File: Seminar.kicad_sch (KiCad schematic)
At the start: 17 parts, among them SW1 SW_Push, SW2 SW_Push, U1 NUCLEO64-F446RE, U2 PCF8574AP

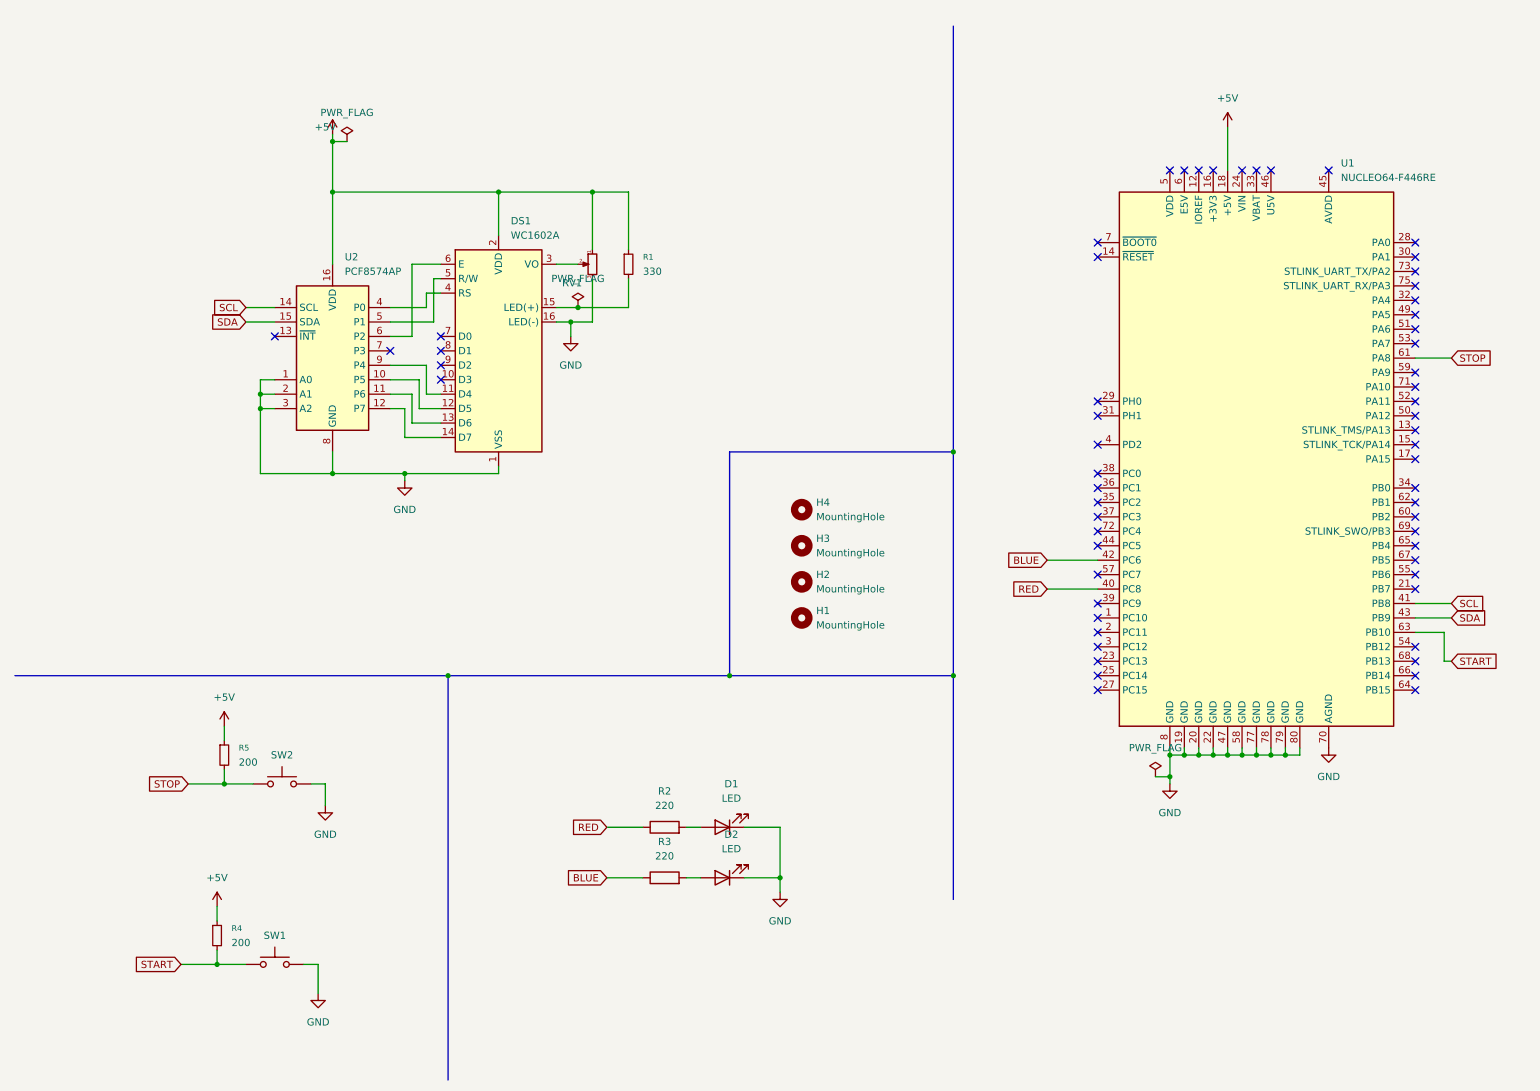
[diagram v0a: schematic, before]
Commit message: Update Seminar 7.12.
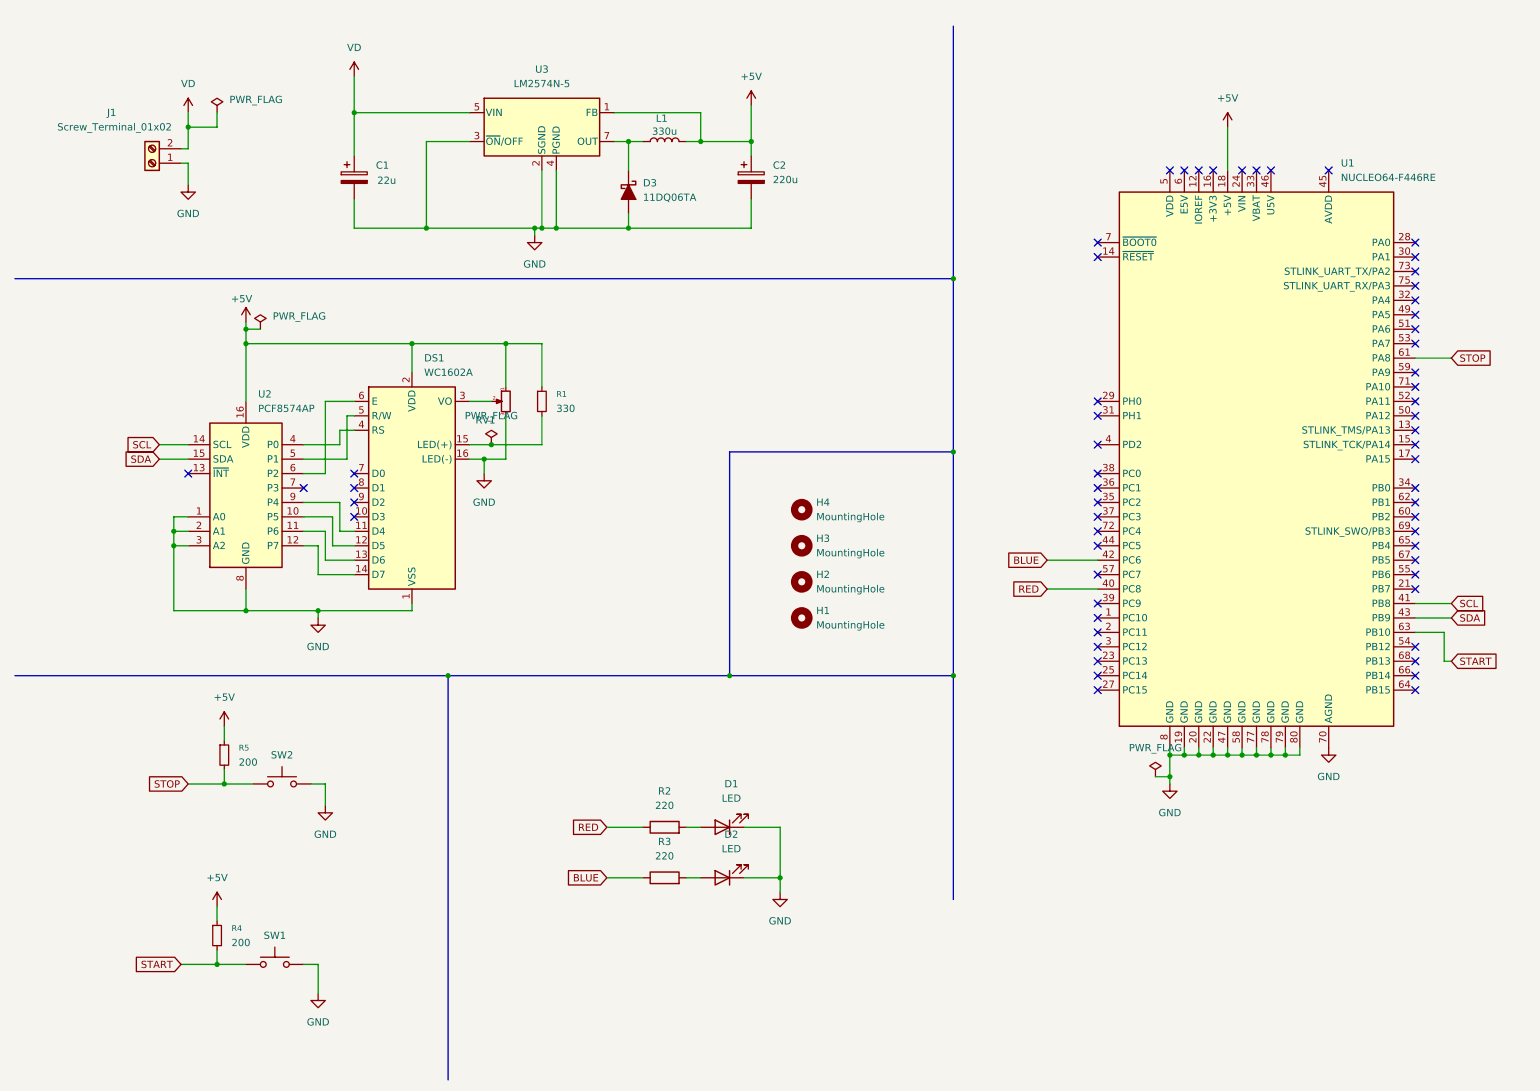
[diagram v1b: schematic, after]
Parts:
- added C1: 22u, Capacitor_THT:CP_Radial_D5.0mm_P2.00mm, symbol Device:C_Polarized
- added C2: 220u, Capacitor_THT:CP_Radial_D5.0mm_P2.00mm, symbol Device:C_Polarized
- added D3: 11DQ06TA, Diode_THT:D_DO-41_SOD81_P12.70mm_Horizontal, symbol Device:D_Schottky_Filled
- added J1: Screw_Terminal_01x02, TerminalBlock_MetzConnect:TerminalBlock_MetzConnect_Type011_RT05502HBLC_1x02_P5.00mm_Horizontal, symbol Connector:Screw_Terminal_01x02
- added L1: 330u, Inductor_THT:L_Radial_D7.2mm_P3.00mm_Murata_1700, symbol Device:L
- added U3: LM2574N-5, Package_DIP:DIP-8_W7.62mm, symbol Regulator_Switching:LM2574N-5
- DS1: Manufacturer (none) -> Wandisplay; Manufacturer part number (none) -> WC1602B0SGW6B-A1
- U1: Manufacturer (none) -> STMicroelectronics; Manufacturer part number (none) -> STM32F446RET6
- U2: Manufacturer (none) -> NXP; Manufacturer part number (none) -> PCF8574AP,112
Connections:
- net +5V: now also C2.1, L1.2, U3.1 (FB)
- net GND: now also C1.2, C2.2, D3.2 (A), J1.1 (Pin_1), U3.2 (SGND), U3.3 (~{ON}/OFF), U3.4 (PGND)
- new net: D3.1 (K), L1.1, U3.7 (OUT)
- new net VD: C1.1, J1.2 (Pin_2), U3.5 (VIN)
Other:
- moved on the sheet: DS1, R1, RV1, U2

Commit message: Update Seminar 7.12. dva
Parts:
- RV1: footprint Potentiometer_SMD:Potentiometer_ACP_CA6-VSMD_Vertical -> Potentiometer_THT:Potentiometer_Bourns_3299Y_Vertical
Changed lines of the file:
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@@
 			)
 		)
-		(property "Footprint" "Potentiometer_SMD:Potentiometer_ACP_CA6-VSMD_Vertical"
+		(property "Footprint" "Potentiometer_THT:Potentiometer_Bourns_3299Y_Vertical"
 			(at 99.06 78.74 0)
 			(effects

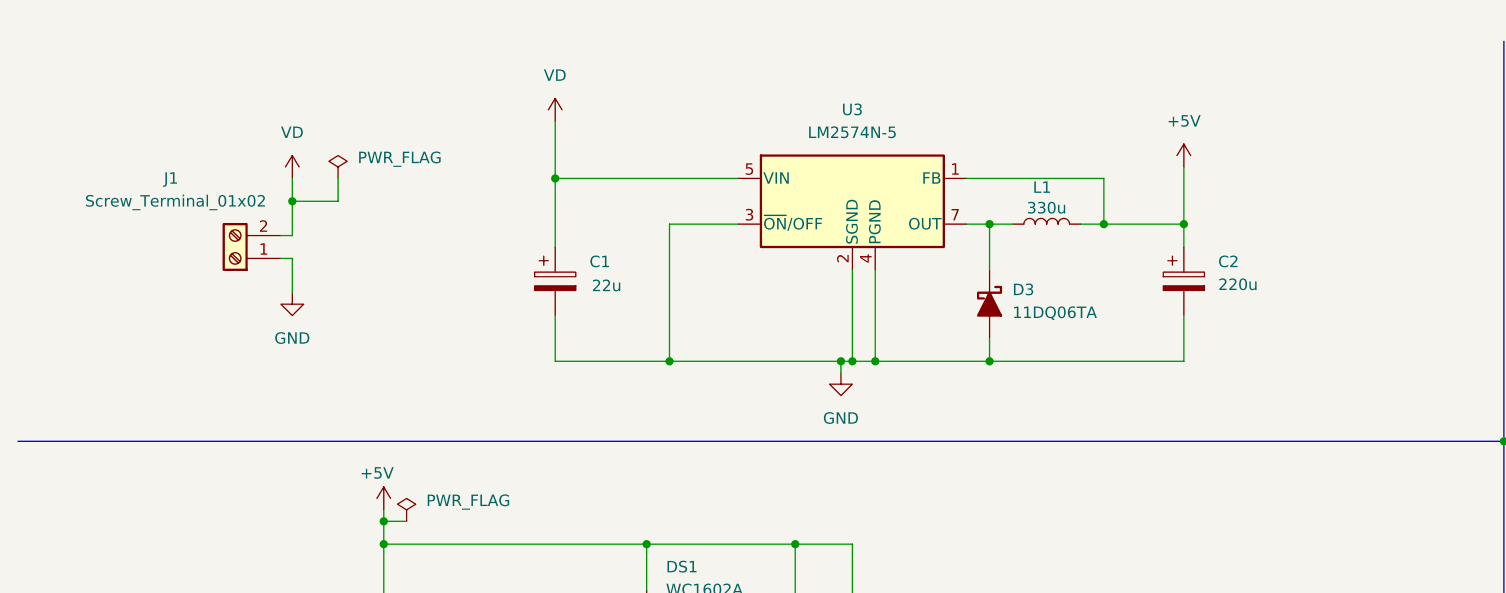
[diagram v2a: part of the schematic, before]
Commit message: Baterija i Step up
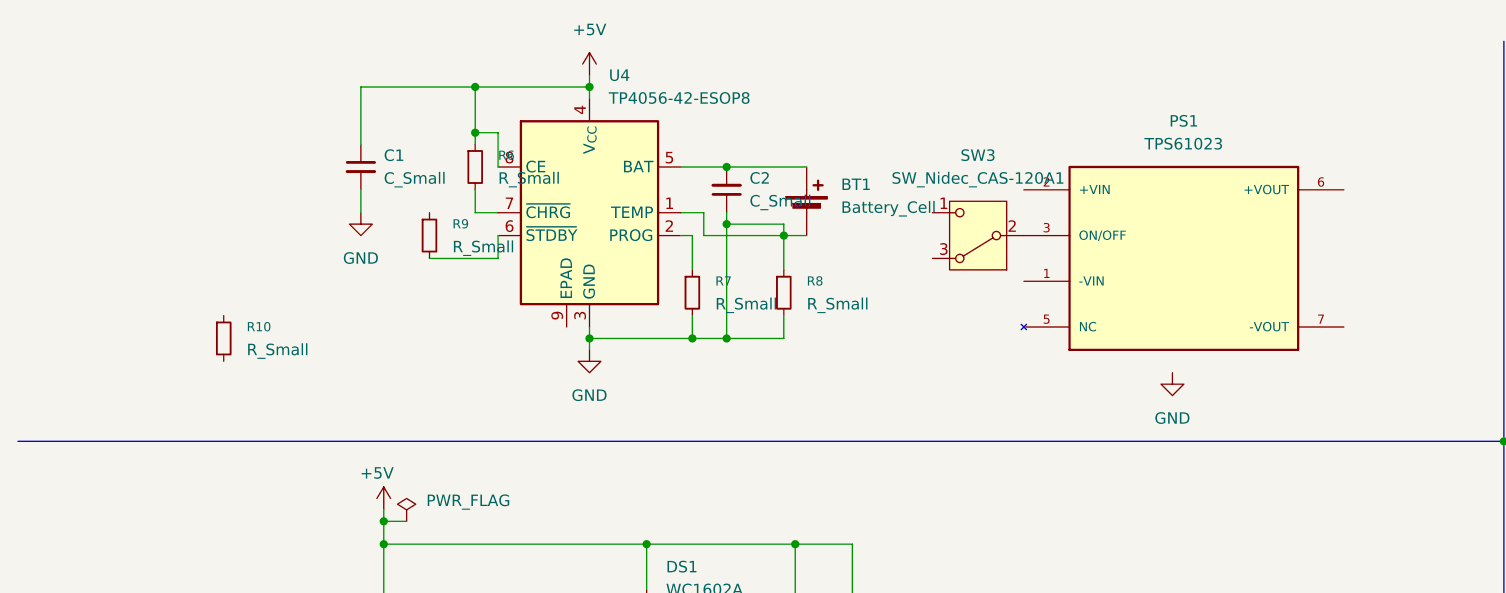
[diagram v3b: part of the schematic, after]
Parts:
- removed C1: 22u, Capacitor_THT:CP_Radial_D5.0mm_P2.00mm, symbol Device:C_Polarized
- removed C2: 220u, Capacitor_THT:CP_Radial_D5.0mm_P2.00mm, symbol Device:C_Polarized
- removed D3: 11DQ06TA, Diode_THT:D_DO-41_SOD81_P12.70mm_Horizontal, symbol Device:D_Schottky_Filled
- removed J1: Screw_Terminal_01x02, TerminalBlock_MetzConnect:TerminalBlock_MetzConnect_Type011_RT05502HBLC_1x02_P5.00mm_Horizontal, symbol Connector:Screw_Terminal_01x02
- removed L1: 330u, Inductor_THT:L_Radial_D7.2mm_P3.00mm_Murata_1700, symbol Device:L
- removed U3: LM2574N-5, Package_DIP:DIP-8_W7.62mm, symbol Regulator_Switching:LM2574N-5
- added BT1: Battery_Cell, symbol Device:Battery_Cell
- added C1, C2: C_Small, symbol Device:C_Small
- added PS1: TPS61023, CONV_PDQ2-D5-S3-S:CONV_PDQ2-D5-S3-S, symbol PDQ2-D5-S3-S:PDQ2-D5-S3-S
- added R10, R6, R7, R8, R9: R_Small, symbol Device:R_Small
- added SW3: SW_Nidec_CAS-120A1, Button_Switch_SMD:Nidec_Copal_CAS-120A, symbol Switch:SW_Nidec_CAS-120A1
- added U4: TP4056-42-ESOP8, Package_SO:SOIC-8-1EP_3.9x4.9mm_P1.27mm_EP2.41x3.3mm_ThermalVias, symbol Battery_Management:TP4056-42-ESOP8
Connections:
- net +5V: now also C1.1, R6.1, U4.4 (V_{CC}), U4.8 (CE)
- net GND: now also BT1.2 (-), C1.2, C2.1, R7.2, R8.1, R8.2, U4.1 (TEMP), U4.3 (GND)
- new net: R7.1, U4.2 (PROG)
- new net: BT1.1 (+), C2.2, U4.5 (BAT)
- new net: R9.2, U4.6 (~{STDBY})
- new net: R6.2, U4.7 (~{CHRG})
- new net: PS1.3 (ON/OFF), SW3.2 (B)
- new net: PS1.5 (NC), PS1.8 (NC)
